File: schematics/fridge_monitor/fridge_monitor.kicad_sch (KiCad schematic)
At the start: 6 parts, among them U1 ESP8266EX, U2 DHT11

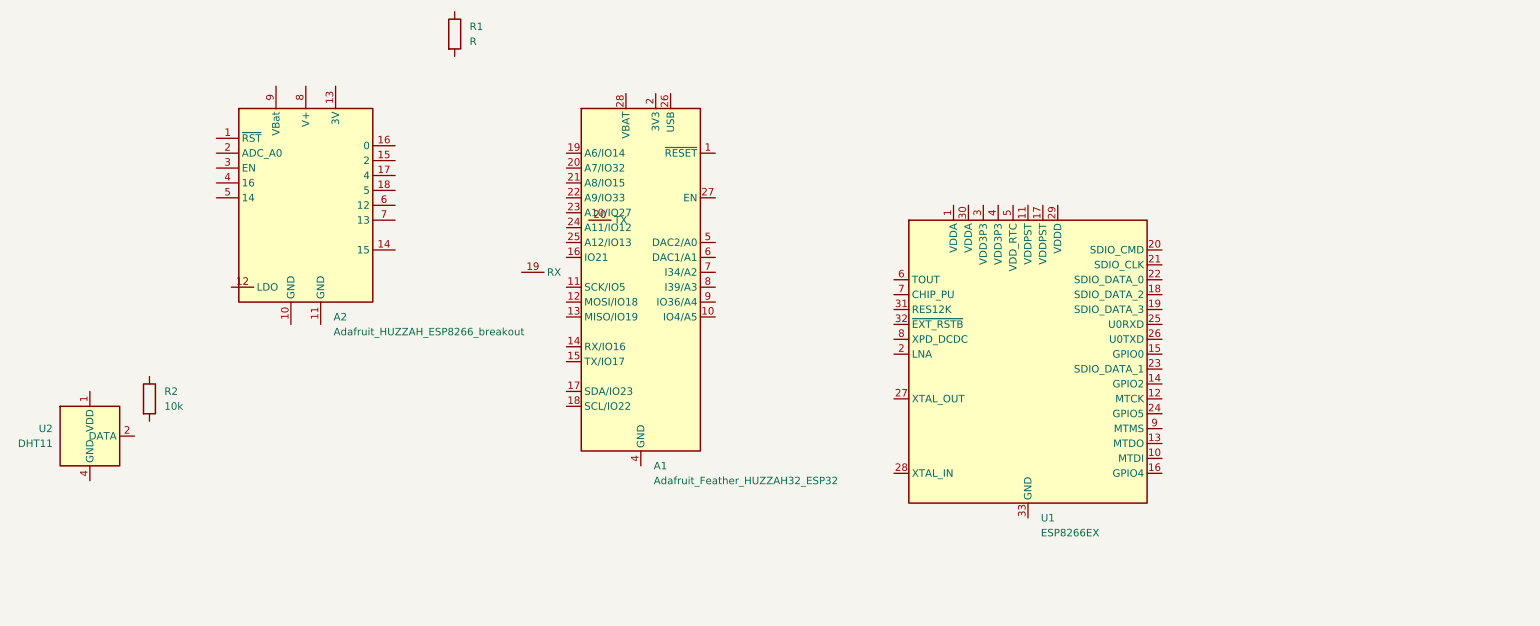
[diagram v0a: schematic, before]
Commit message: initial_schematic
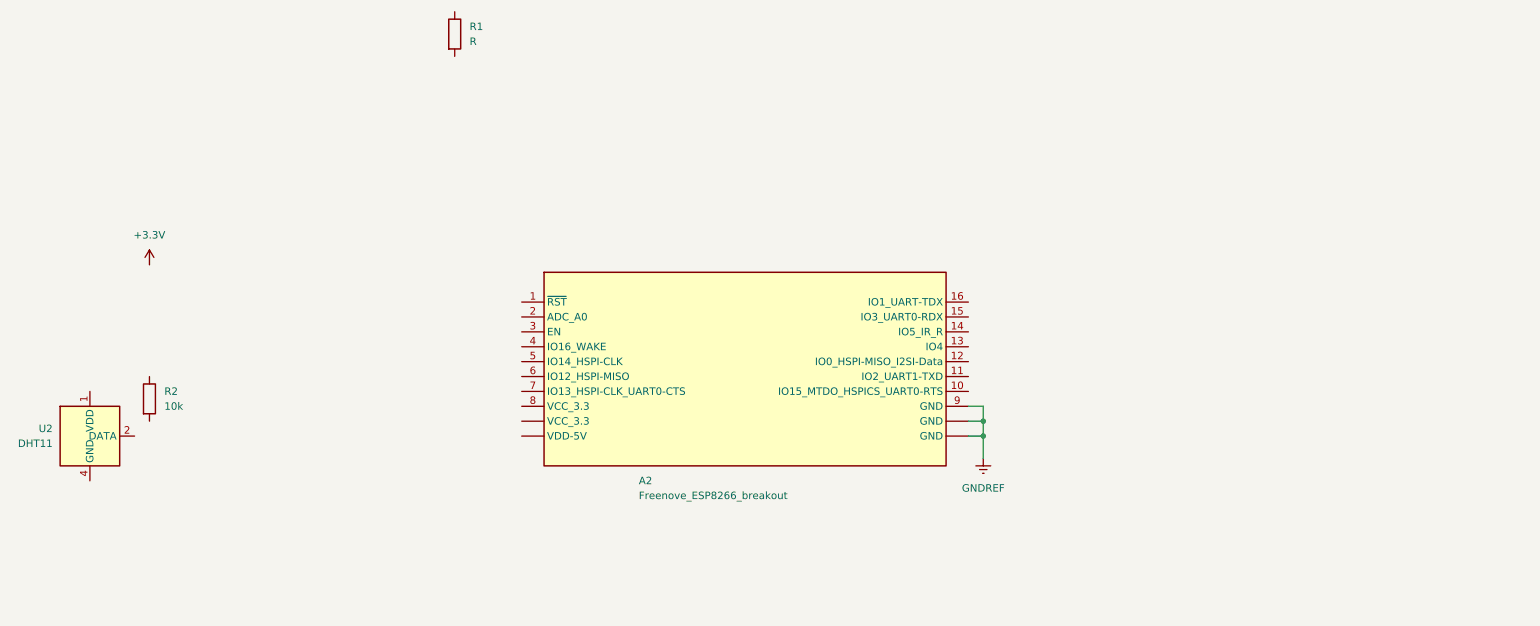
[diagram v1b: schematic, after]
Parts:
- removed A1: Adafruit_Feather_HUZZAH32_ESP32, Module:Adafruit_Feather, symbol MCU_Module:Adafruit_Feather_HUZZAH32_ESP32
- removed U1: ESP8266EX, Package_DFN_QFN:QFN-32-1EP_5x5mm_P0.5mm_EP3.45x3.45mm, symbol MCU_Espressif:ESP8266EX
- A2: value Adafruit_HUZZAH_ESP8266_breakout -> Freenove_ESP8266_breakout
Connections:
- net GNDREF: now reaches A2.9 (GND)
- net GNDREF: now also A2. (VDD-5V)
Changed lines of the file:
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@@
 (kicad_sch (version 20230121) (generator eeschema)
   (paper "A4")
-  (symbol (lib_id "MCU_Module:Adafruit_HUZZAH_ESP8266_breakout") (at 76.2 63.5 0) (unit 1)
+  (junction (at 191.77 102.87) (diameter 0) (color 0 0 0 0)
+  )
+  (junction (at 191.77 100.33) (diameter 0) (color 0 0 0 0)
+  )
+  (wire (pts (xy 191.77 102.87) (xy 189.23 102.87))
+    (stroke (width 0) (type default))
+  )
+  (wire (pts (xy 189.23 97.79) (xy 191.77 97.79))
+    (stroke (width 0) (type default))
+  )
+  (wire (pts (xy 191.77 100.33) (xy 191.77 102.87))
+    (stroke (width 0) (type default))
+  )
+  (wire (pts (xy 191.77 106.68) (xy 191.77 102.87))
+    (stroke (width 0) (type default))
+  )
+  (wire (pts (xy 191.77 97.79) (xy 191.77 100.33))
+    (stroke (width 0) (type default))
+  )
+  (wire (pts (xy 189.23 100.33) (xy 191.77 100.33))
+    (stroke (width 0) (type default))
+  )
+  (symbol (lib_id "power:+3.3V") (at 49.53 73.66 0) (unit 1)
     (in_bom yes) (on_board yes) (dnp no) (fields_autoplaced)
-    (property "Reference" "A2" (at 80.9341 82.55 0)
+    (property "Reference" "#PWR01" (at 49.53 77.47 0)
+      (effects (font (size 1.27 1.27)) hide)
+    )
+    (property "Value" "+3.3V" (at 49.53 68.58 0)
+      (effects (font (size 1.27 1.27)))
+    )
+    (property "Footprint" "" (at 49.53 73.66 0)
+      (effects (font (size 1.27 1.27)) hide)
+    )
+    (property "Datasheet" "" (at 49.53 73.66 0)
+      (effects (font (size 1.27 1.27)) hide)
+    )
+    (pin "1")
+    (instances
+      (project "fridge_monitor"
+        (path "/4a0a8a0e-076c-4b7e-886e-1c07c60b99a2"
+          (reference "#PWR01") (unit 1)
+        )
+      )
+    )
+  )
+  (symbol (lib_id "MCU_Module:Adafruit_HUZZAH_ESP8266_breakout") (at 128.27 91.44 0) (unit 1)
+    (in_bom yes) (on_board yes) (dnp no) (fields_autoplaced)
+    (property "Reference" "A2" (at 133.0041 110.49 0)
       (effects (font (size 1.27 1.27)) (justify left))
     )
-    (property "Value" "Adafruit_HUZZAH_ESP8266_breakout" (at 80.9341 85.09 0)
+    (property "Value" "Freenove_ESP8266_breakout" (at 133.0041 113.03 0)
       (effects (font (size 1.27 1.27)) (justify left))
     )
-    (property "Footprint" "" (at 81.28 48.26 0)
+    (property "Footprint" "" (at 133.35 76.2 0)
       (effects (font (size 1.27 1.27)) hide)
     )
-    (property "Datasheet" "https://www.adafruit.com/product/2471" (at 83.82 45.72 0)
+    (property "Datasheet" "" (at 135.89 73.66 0)
       (effects (font (size 1.27 1.27)) hide)
     )
-    (pin "19")
+    (pin "")
     (pin "2")
     (pin "6")
     (pin "14")
-    (pin "18")
+    (pin "")
     (pin "13")
     (pin "3")
     (pin "12")
     (pin "1")
-    (pin "17")
+    (pin "")
     (pin "10")
-    (pin "20")
+    (pin "")
     (pin "4")
     (pin "5")
@@
     )
   )
-  (symbol (lib_id "MCU_Espressif:ESP8266EX") (at 199.39 88.9 0) (unit 1)
+  (symbol (lib_id "power:GNDREF") (at 191.77 106.68 0) (unit 1)
     (in_bom yes) (on_board yes) (dnp no) (fields_autoplaced)
-    (property "Reference" "U1" (at 201.5841 116.84 0)
-      (effects (font (size 1.27 1.27)) (justify left))
-    )
-    (property "Value" "ESP8266EX" (at 201.5841 119.38 0)
-      (effects (font (size 1.27 1.27)) (justify left))
-    )
-    (property "Footprint" "Package_DFN_QFN:QFN-32-1EP_5x5mm_P0.5mm_EP3.45x3.45mm" (at 199.39 121.92 0)
+    (property "Reference" "#PWR02" (at 191.77 113.03 0)
       (effects (font (size 1.27 1.27)) hide)
     )
-    (property "Datasheet" "http://espressif.com/sites/default/files/documentation/0a-esp8266ex_datasheet_en.pdf" (at 201.93 121.92 0)
+    (property "Value" "GNDREF" (at 191.77 111.76 0)
+      (effects (font (size 1.27 1.27)))
+    )
+    (property "Footprint" "" (at 191.77 106.68 0)
       (effects (font (size 1.27 1.27)) hide)
     )
-    (pin "5")
-    (pin "4")
-    (pin "18")
-    (pin "27")
-    (pin "8")
-    (pin "26")
-    (pin "6")
-    (pin "7")
-    (pin "29")
-    (pin "32")
-    (pin "22")
-    (pin "10")
-    (pin "12")
+    (property "Datasheet" "" (at 191.77 106.68 0)
+      (effects (font (size 1.27 1.27)) hide)
+    )
     (pin "1")
-    (pin "13")
-    (pin "20")
-    (pin "11")
-    (pin "31")
-    (pin "24")
-    (pin "21")
-    (pin "3")
-    (pin "25")
-    (pin "30")
-    (pin "2")
-    (pin "16")
-    (pin "28")
-    (pin "33")
-    (pin "23")
-    (pin "19")
-    (pin "17")
-    (pin "9")
-    (pin "15")
-    (pin "14")
     (instances
       (project "fridge_monitor"
         (path "/4a0a8a0e-076c-4b7e-886e-1c07c60b99a2"
-          (reference "U1") (unit 1)
+          (reference "#PWR02") (unit 1)
         )
       )
@@
         )
       )
-    )
-  )
-  (symbol (lib_id "MCU_Module:Adafruit_Feather_HUZZAH32_ESP32") (at 133.35 74.93 0) (unit 1)
-    (in_bom yes) (on_board yes) (dnp no) (fields_autoplaced)
-    (property "Reference" "A1" (at 135.5441 107.95 0)
-      (effects (font (size 1.27 1.27)) (justify left))
-    )
-    (property "Value" "Adafruit_Feather_HUZZAH32_ESP32" (at 135.5441 110.49 0)
-      (effects (font (size 1.27 1.27)) (justify left))
-    )
-    (property "Footprint" "Module:Adafruit_Feather" (at 135.89 109.22 0)
-      (effects (font (size 1.27 1.27)) (justify left) hide)
-    )
-    (property "Datasheet" "https://cdn-learn.adafruit.com/downloads/pdf/adafruit-huzzah32-esp32-feather.pdf" (at 133.35 105.41 0)
-      (effects (font (size 1.27 1.27)) hide)
-    )
-    (pin "20")
-    (pin "6")
-    (pin "27")
-    (pin "19")
-    (pin "9")
-    (pin "4")
-    (pin "1")
-    (pin "12")
-    (pin "2")
-    (pin "3")
-    (pin "23")
-    (pin "28")
-    (pin "17")
-    (pin "18")
-    (pin "25")
-    (pin "7")
-    (pin "24")
-    (pin "5")
-    (pin "26")
-    (pin "10")
-    (pin "14")
-    (pin "15")
-    (pin "11")
-    (pin "13")
-    (pin "16")
-    (pin "21")
-    (pin "22")
-    (pin "8")
-    (instances
-      (project "fridge_monitor"
-        (path "/4a0a8a0e-076c-4b7e-886e-1c07c60b99a2"
-          (reference "A1") (unit 1)
-        )
-      )

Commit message: initial_schematic
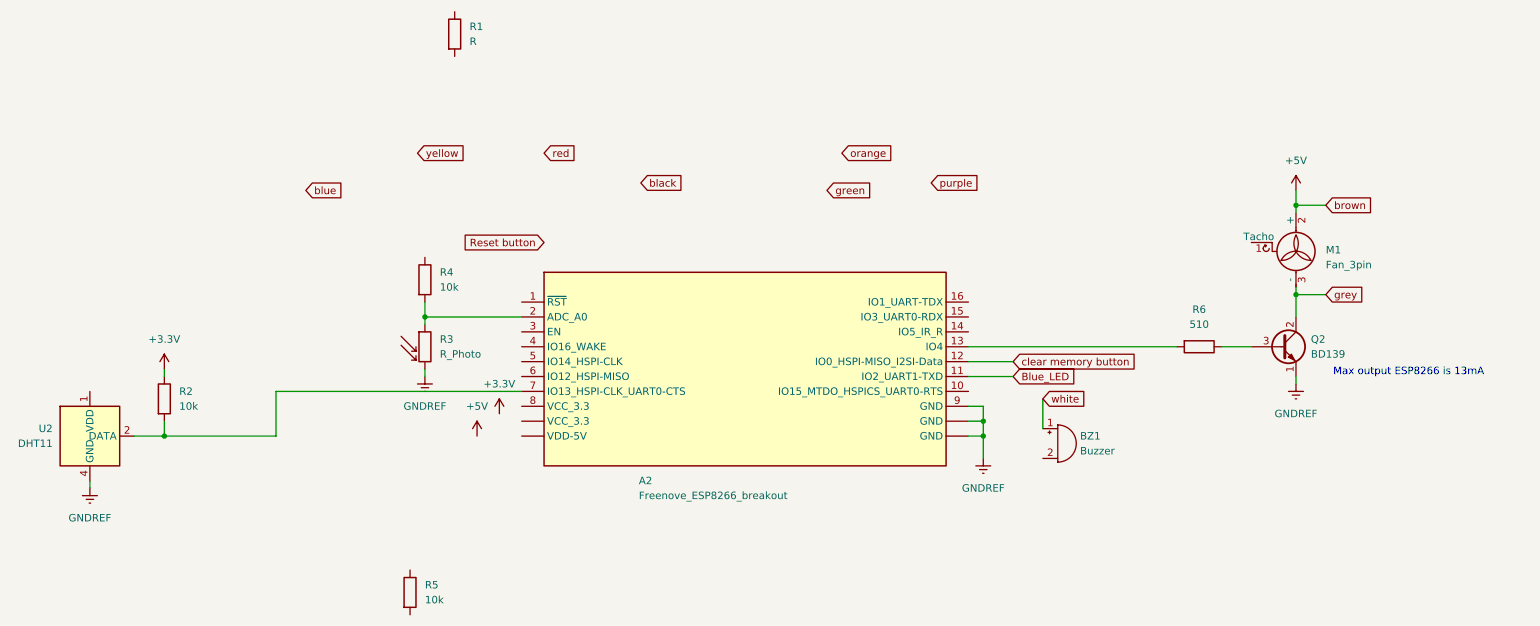
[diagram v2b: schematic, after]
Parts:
- added BZ1: Buzzer, symbol Device:Buzzer
- added M1: Fan_3pin, symbol Motor:Fan_3pin
- added Q2: BD139, Package_TO_SOT_THT:TO-126-3_Vertical, symbol Transistor_BJT:BD139
- added R3: R_Photo, symbol Device:R_Photo
- added R4, R5: 10k, symbol Device:R
- added R6: 510, symbol Device:R
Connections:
- net +3.3V: now also R2.1
- net GNDREF: now also U2.4 (GND), Q2.1 (E), R3.2
- net Blue_LED: now reaches A2.11 (IO2_UART1-TXD)
- net clear memory button: now reaches A2.12 (IO0_HSPI-MISO_I2SI-Data)
- net at A2.13 (IO4): now also R6.2
- net at A2.2 (ADC_A0): now also R3.1, R4.2
- net at A2.7 (IO13_HSPI-CLK_UART0-CTS): now also R2.2, U2.2 (DATA)
- new net: Q2.3 (B), R6.1
- new net +5V: M1.2 (+)
- new net grey: M1.3 (-), Q2.2 (C)
- new net white: BZ1.1 (+)
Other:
- note added: "Max output ESP8266 is 13mA"
- moved on the sheet: R2
